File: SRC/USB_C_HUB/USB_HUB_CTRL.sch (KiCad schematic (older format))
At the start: 27 parts

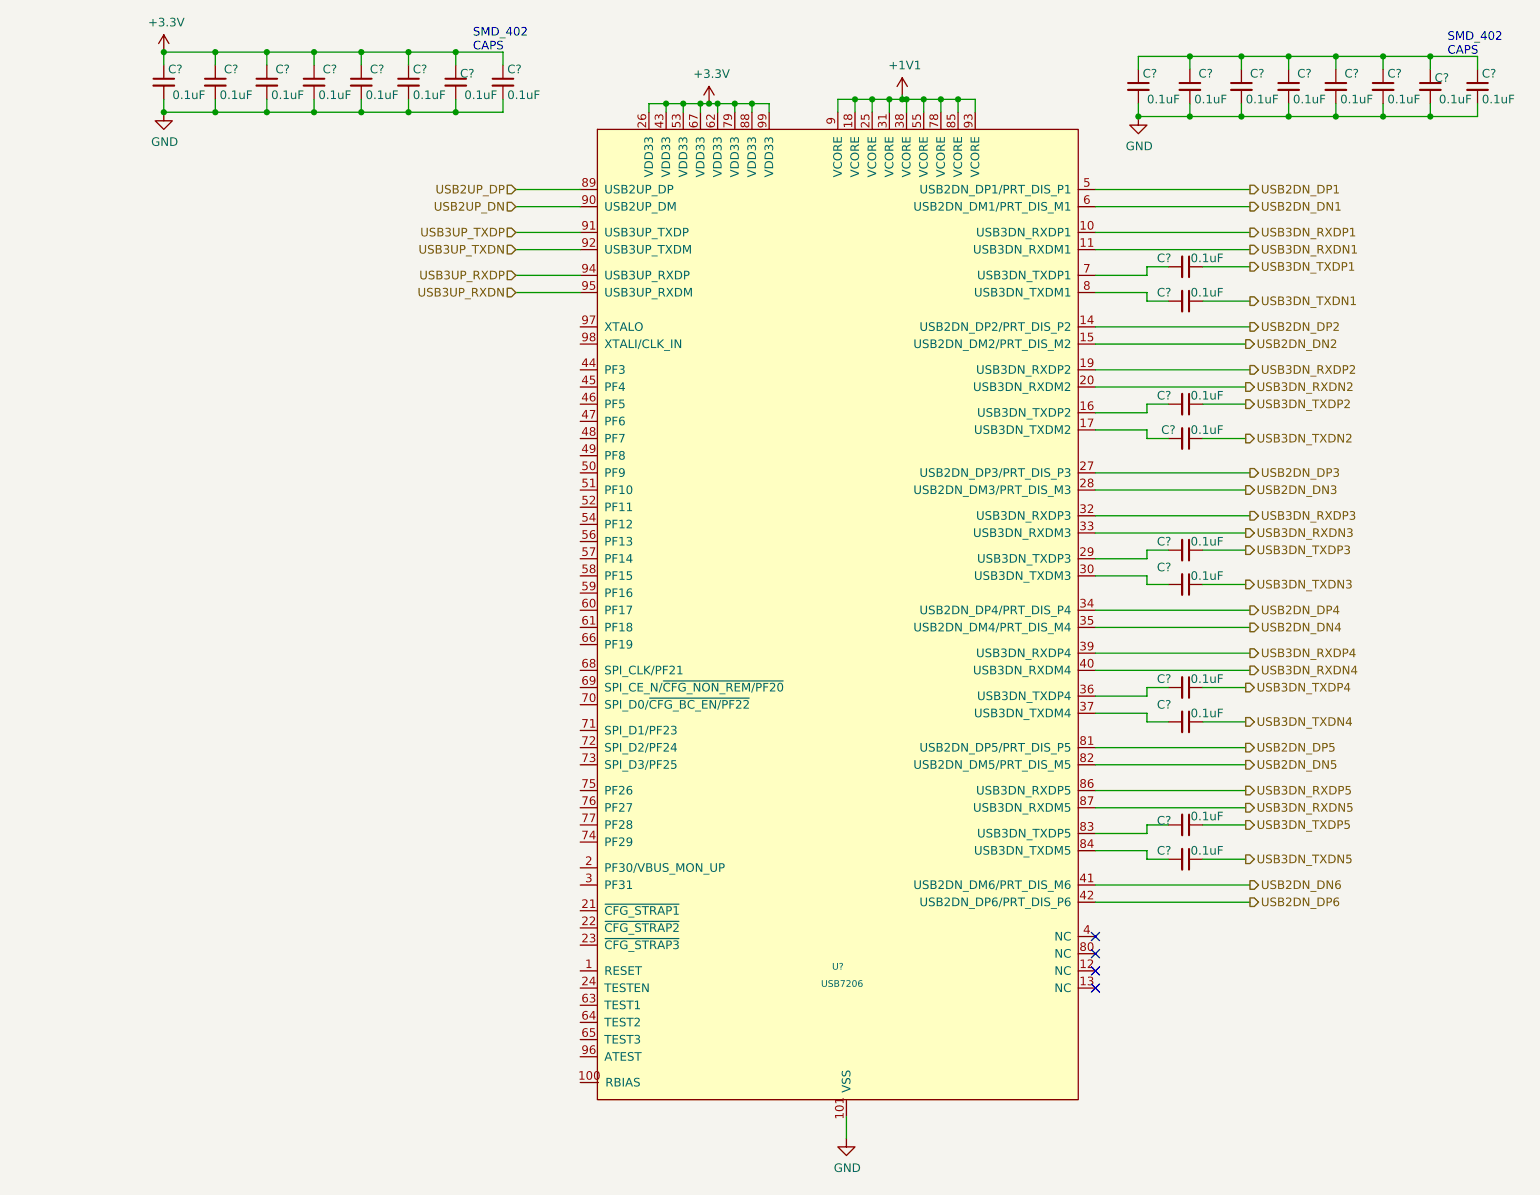
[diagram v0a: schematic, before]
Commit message: commit with all DFPs properly connected
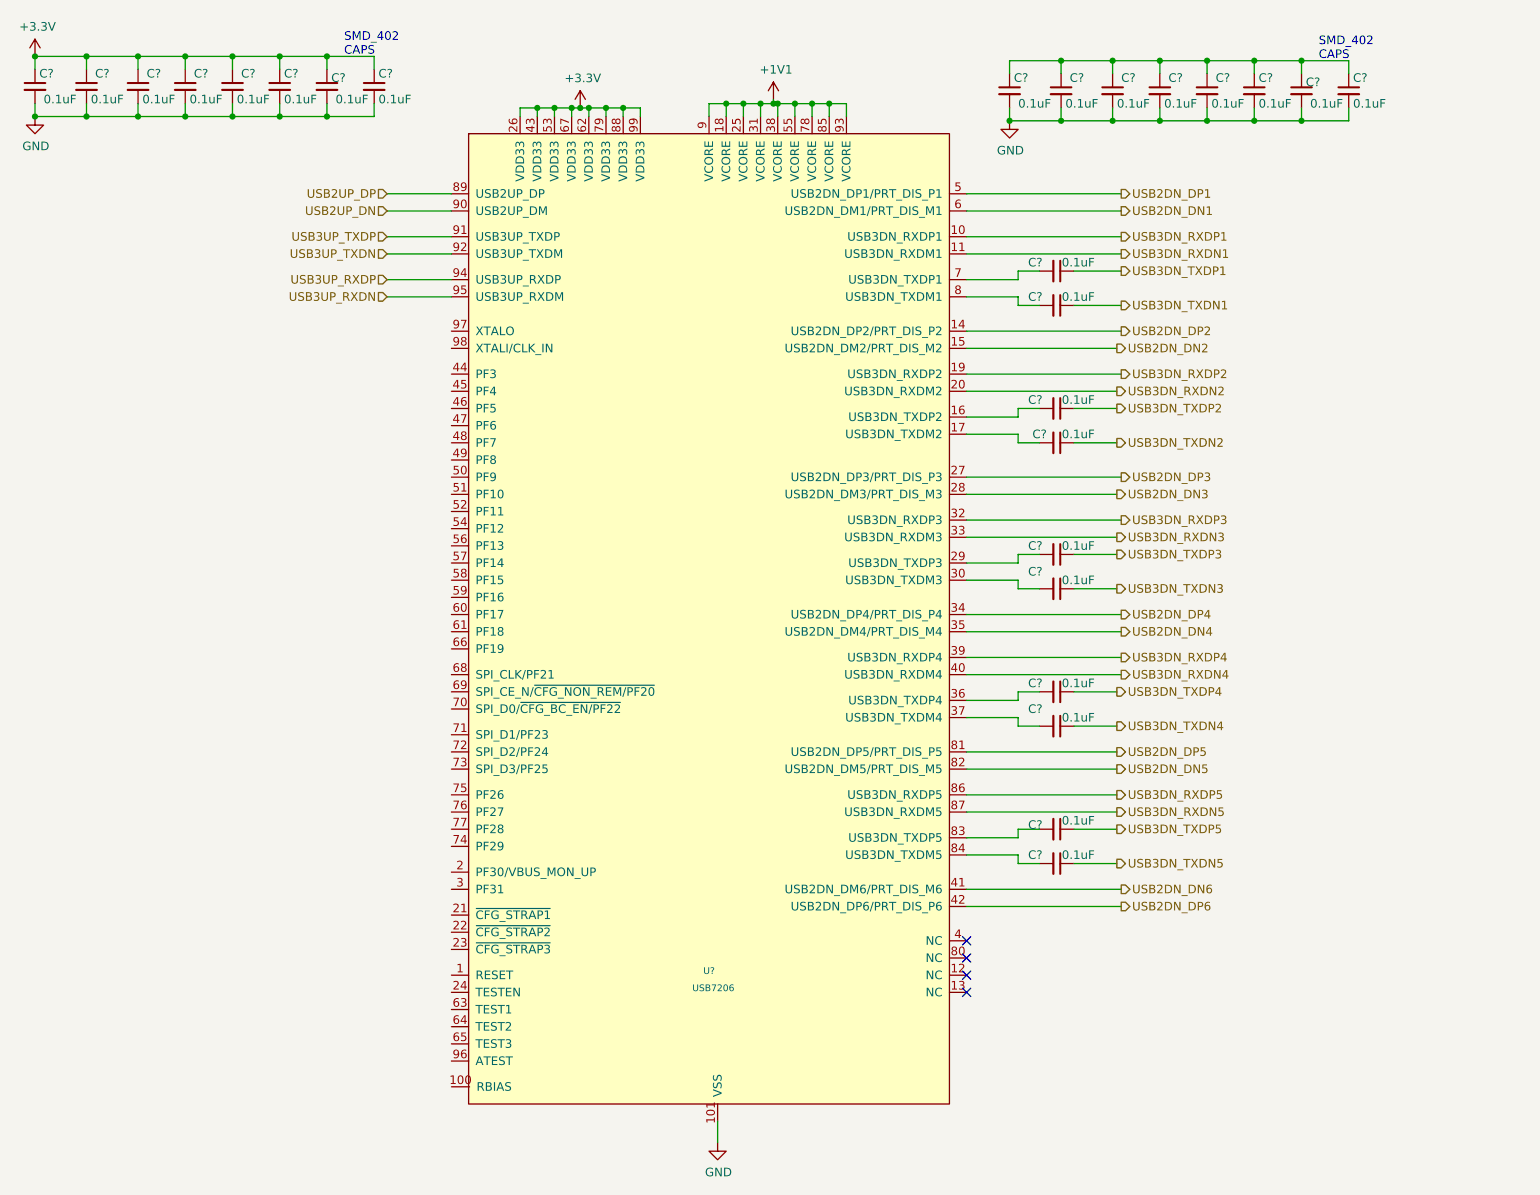
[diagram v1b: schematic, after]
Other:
- moved on the sheet: C?, U?
